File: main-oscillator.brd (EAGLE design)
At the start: 89.8 x 26.7 mm, 14 parts, among them IC1 7805TV, IC2 UA555N

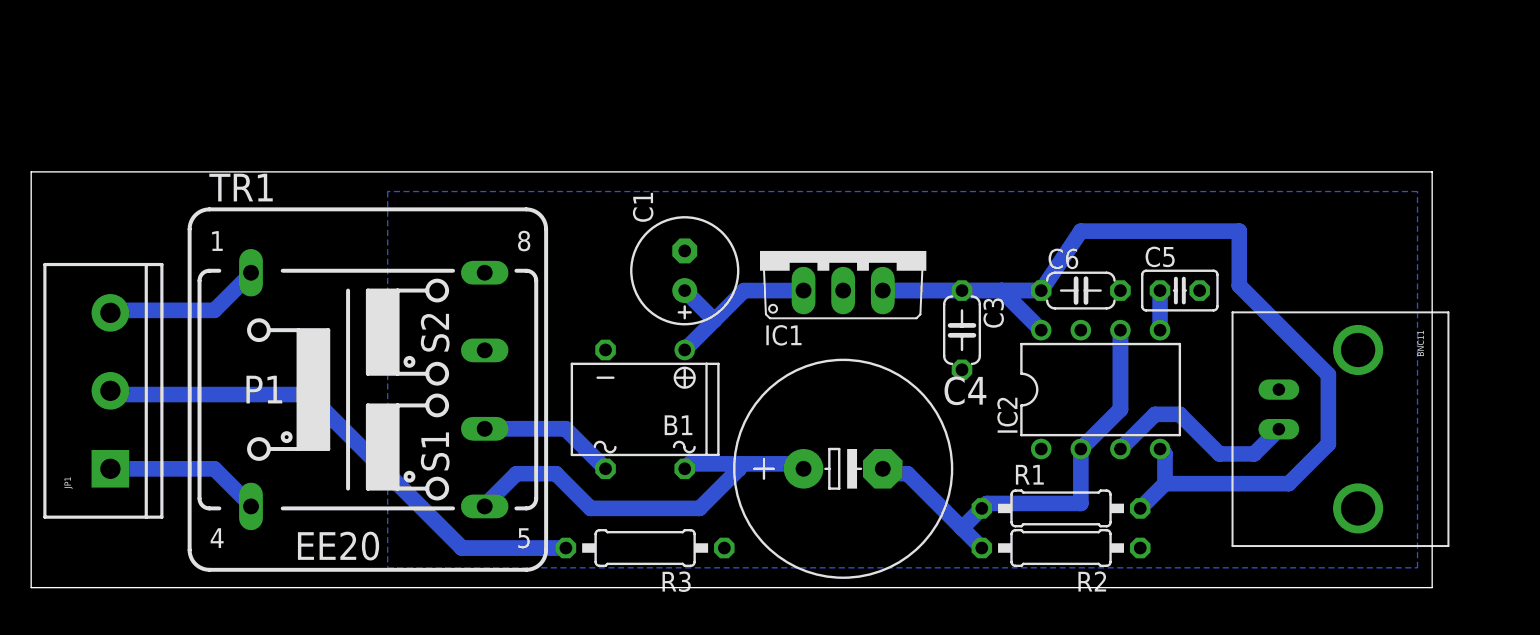
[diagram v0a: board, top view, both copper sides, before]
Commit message: v 1.1: added switch gitignore updated with 'stuff' folder
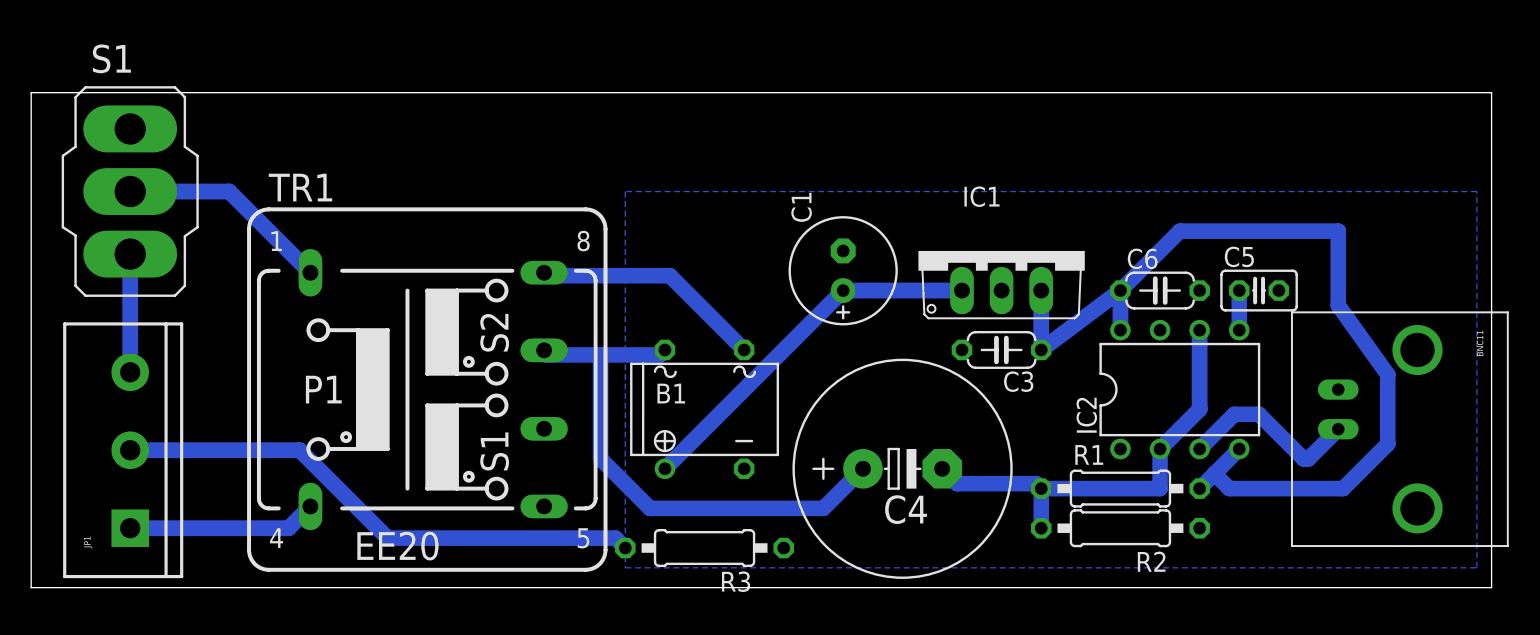
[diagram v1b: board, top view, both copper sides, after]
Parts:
- added S1: (no value), switch:320-916
- moved C1 10.2 mm to (52.1, 20.3)
- moved IC1 10.2 mm to (62.2, 21.6)
- moved C5 5.08 mm to (78.7, 19.1)
- moved C6 5.08 mm to (72.4, 19.1)
- moved IC2 5.08 mm to (73.7, 12.7)
- moved JP1 4.02 mm to (6.35, 3.81)
- moved R1 4.02 mm to (69.8, 6.35)
- moved R2 4.02 mm to (69.8, 3.81)
- moved B1 3.81 mm to (43.2, 11.4), turned to 0 degrees
- moved C4 3.81 mm to (55.9, 7.62)
- moved R3 3.81 mm to (43.2, 2.54)
- moved TR1 3.81 mm to (25.4, 12.7)
- moved BNC11 3.81 mm to (83.8, 10.2)
- moved C3 2.84 mm to (62.2, 15.2), turned to 180 degrees
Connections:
- new net N$10: JP1.3, S1.3
- net N$1: now also S1.2; no longer JP1.3
- net N$2: now also TR1.7; no longer TR1.5
- net N$6: now also TR1.8; no longer TR1.6
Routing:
- net N$5: track 11.9 -> 23.8 mm
- net N$10: track 0.00 -> 7.58 mm
- net N$2: track 27.4 -> 33.9 mm
- net N$6: track 8.81 -> 14.9 mm
- net N$1: track 10.2 -> 13.7 mm
- net N$3: track 10.0 -> 12.4 mm
- net V+: track 60.6 -> 59.2 mm
- net N$9: track 12.8 -> 11.8 mm
- net N$4: track 33.5 -> 34.3 mm
- net N$8: track 28.9 -> 28.2 mm
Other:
- board size 89.8 x 26.7 mm -> 93.7 x 31.7 mm
